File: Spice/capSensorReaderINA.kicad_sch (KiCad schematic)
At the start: 22 parts, among them U1 LM358, U2 LM358

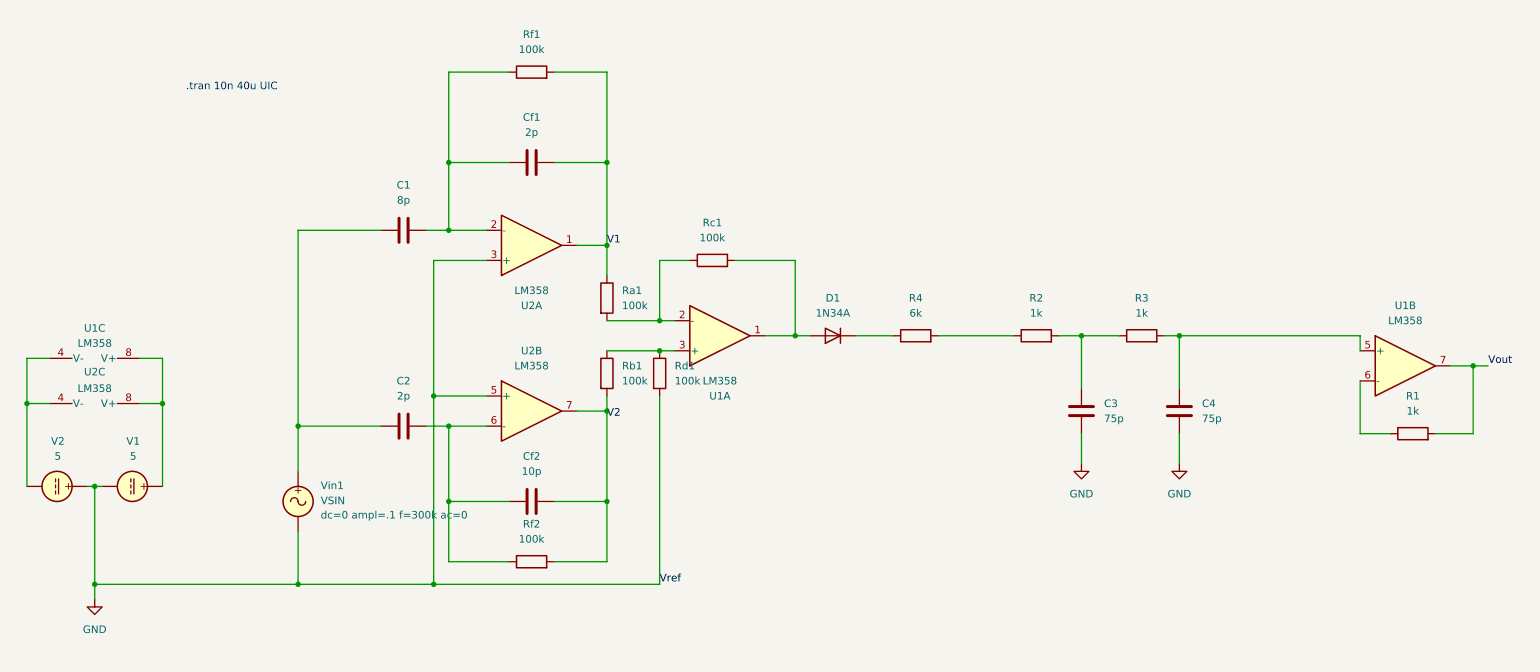
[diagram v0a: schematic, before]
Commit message: Better Sensor Reader
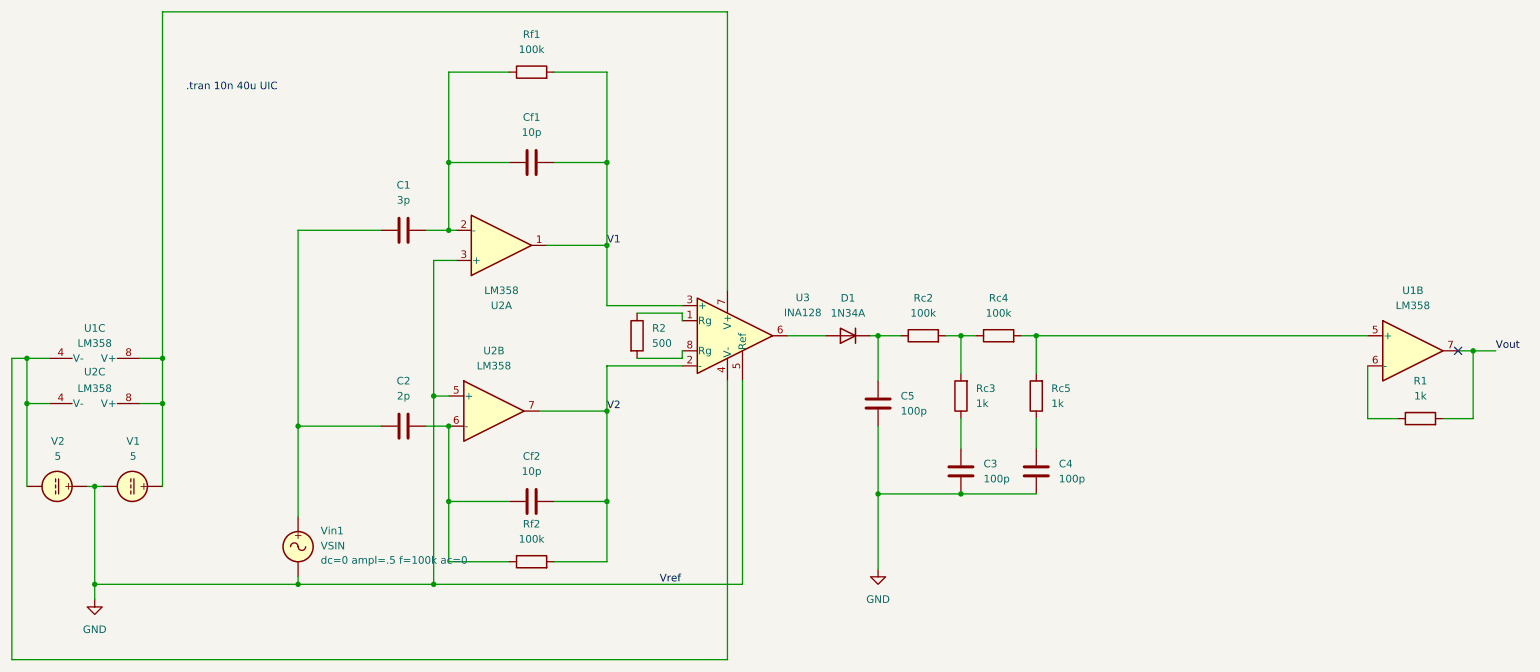
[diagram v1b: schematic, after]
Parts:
- removed R3: 1k, symbol Device:R
- removed R4: 6k, symbol Device:R
- removed Ra1, Rb1, Rc1, Rd1: 100k, symbol Device:R
- removed unit 1 of U1
- added C5: 100p, symbol Device:C
- added Rc2, Rc4: 100k, symbol Device:R
- added Rc3, Rc5: 1k, symbol Device:R
- added U3: INA128, symbol Amplifier_Instrumentation:INA128
- C1: value 8p -> 3p
- C3, C4: value 75p -> 100p
- Cf1: value 2p -> 10p
- R2: value 1k -> 500
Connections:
- net GND: now also C5.2, U3.5 (Ref)
- net V1: now also U3.3 (+)
- net V2: now also U3.2 (-)
- net at U1.4 (V-), U2.4 (V-), V2.2: now also U3.4 (V-)
- net at R2.1: now also U3.1 (Rg)
- net at R2.2: now also U3.8 (Rg); no longer C3.1
- net at D1.2 (A): now also U3.6
- net at C4.1: now also Rc5.1; no longer U1.5 (+)
- net at U1.8 (V+), U2.8 (V+), V1.1: now also U3.7 (V+)
- net at D1.1 (K): now also C5.1, Rc2.1
- new net: Rc4.2, Rc5.2, U1.5 (+)
- new net: C3.1, Rc3.1
- new net: Rc2.2, Rc3.2, Rc4.1
- no-connect marks 0 -> 1
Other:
- moved on the sheet: D1, R1, U1B, U2A, U2B, Vin1
